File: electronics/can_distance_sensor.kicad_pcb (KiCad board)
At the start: 4 copper layers, 40.6 x 40.6 mm, 75 parts, among them J1 USB_B_Micro, J2 Conn_ARM_JTAG_SWD_10, J3 Conn_01x04, Q1 IRLML6401, SW1 PTS645SK50SMTR92LFS, U1 USBLC6-2SC6, U2 STM32G431CBUx, U3 TLV75801PDRV, U4 AOZ1280CI, U5 TLV75801PDRV, U6 TCAN1044A-Q1, U7 VL53L3CXV0DH/1, U8 TCA9509DGKR, Y1 Crystal_GND24

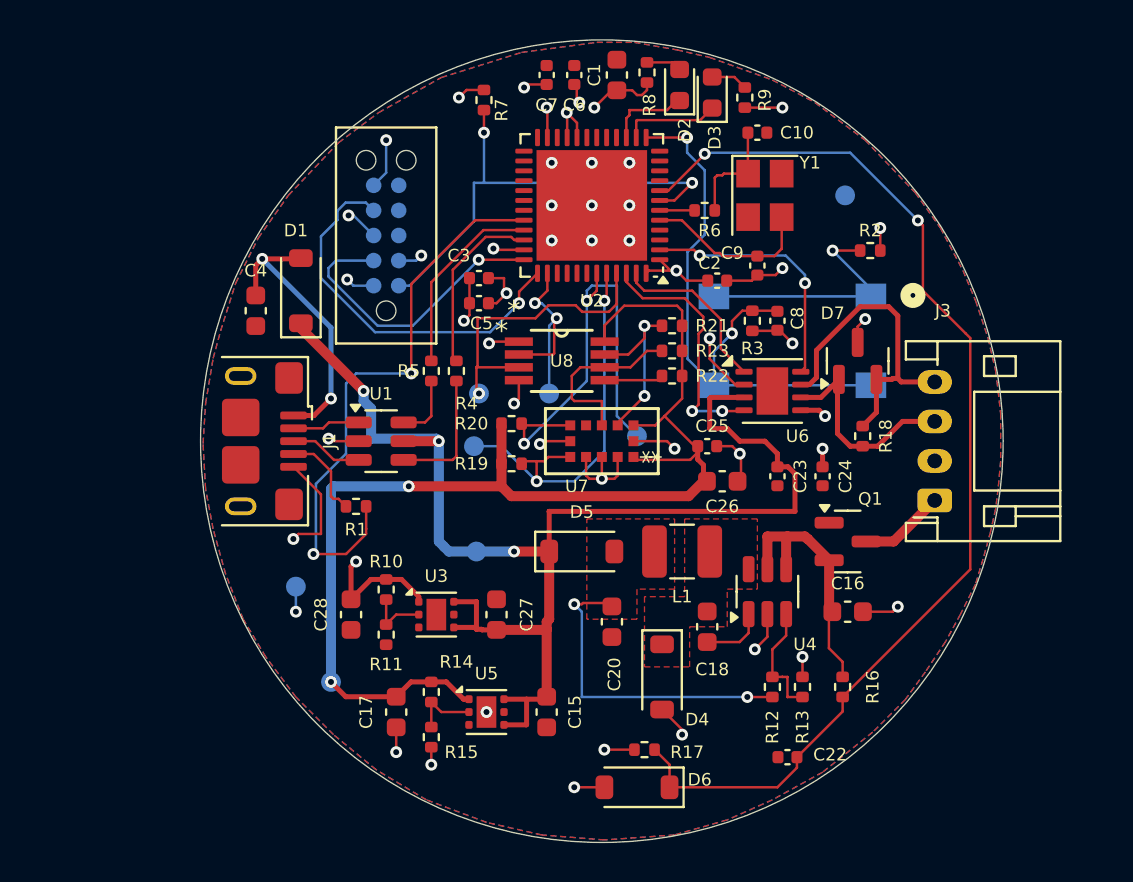
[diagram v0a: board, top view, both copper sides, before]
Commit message: Major refactor to rev B
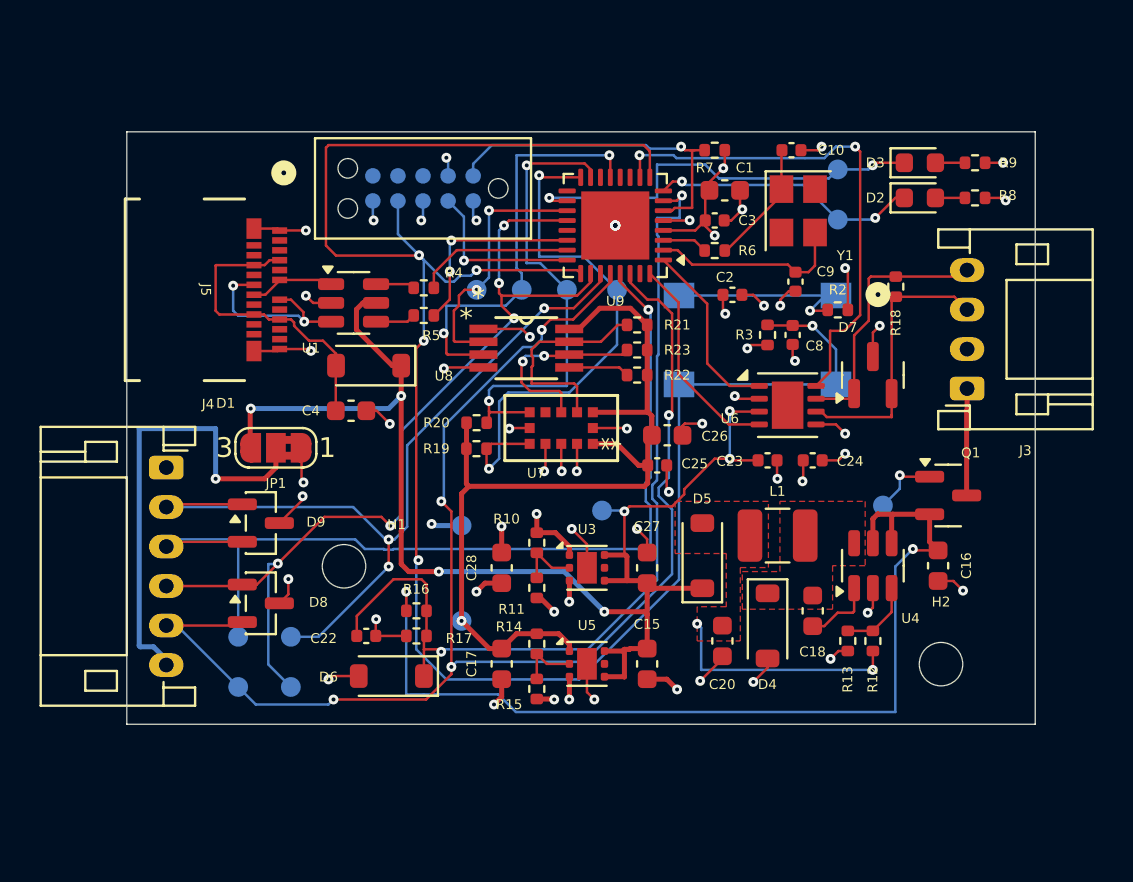
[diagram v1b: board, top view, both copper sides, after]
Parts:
- removed C5, C6, C7: 0.1u, Capacitor_SMD:C_0402_1005Metric
- removed J1: USB_B_Micro, Connector_USB:USB_Micro-B_Amphenol_10118193-0001LF_Horizontal
- removed R1: 560, Resistor_SMD:R_0402_1005Metric
- removed U2: STM32G431CBUx, Package_DFN_QFN:QFN-48-1EP_7x7mm_P0.5mm_EP5.6x5.6mm
- added D8: SP0502BAHT, Package_TO_SOT_SMD:SOT-23, F.Cu at (176.8, 113.9)
- added D9: SP0502BAHT, Package_TO_SOT_SMD:SOT-23, F.Cu at (176.8, 109.8)
- added H1: MountingHole, MountingHole:MountingHole_2.2mm_M2, F.Cu at (181.0, 112.0)
- added H2: MountingHole, MountingHole:MountingHole_2.2mm_M2, F.Cu at (211.2, 117.0)
- added J4: Conn_01x06, Connector_JST:JST_PH_S6B-PH-K_1x06_P2.00mm_Horizontal, F.Cu at (172.0, 107.0)
- added J5: USB_C_Receptacle, footprints:CONN_105450-0101_MOL, F.Cu at (174.0, 98.0)
- added JP1: SolderJumper_3_Bridged12, Jumper:SolderJumper-3_P1.3mm_Bridged2Bar12_RoundedPad1.0x1.5mm_NumberLabels, F.Cu at (177.6, 106.0)
- added TP10: TestPoint, TestPoint:TestPoint_Pad_D1.0mm, B.Cu at (175.6, 115.6)
- added TP11: TestPoint, TestPoint:TestPoint_Pad_D1.0mm, B.Cu at (175.6, 118.1)
- added TP12: TestPoint, TestPoint:TestPoint_Pad_D1.0mm, B.Cu at (178.3, 115.6)
- added TP13: TestPoint, TestPoint:TestPoint_Pad_D1.0mm, B.Cu at (206.0, 94.4)
- added TP14: TestPoint, TestPoint:TestPoint_Pad_D1.0mm, B.Cu at (206.0, 91.9)
- added TP9: TestPoint, TestPoint:TestPoint_Pad_D1.0mm, B.Cu at (178.3, 118.1)
- added U9: STM32G0B1KBUx, Package_DFN_QFN:QFN-32-1EP_5x5mm_P0.5mm_EP3.45x3.45mm, F.Cu at (194.7, 94.7)
- moved C22 22.2 mm to (182.1, 115.5), turned to 0 degrees
- moved TP8 22.1 mm to (190.0, 98.0)
- moved R16 21.9 mm to (184.7, 114.3), turned to 0 degrees
- moved TP1 21.2 mm to (208.3, 108.9), turned to 180 degrees
- moved TP6 20.4 mm to (192.3, 98.0)
- moved R8 17.8 mm to (213.0, 93.3), turned to 0 degrees
- moved D6 13.7 mm to (183.4, 117.6)
- moved D2 13.4 mm to (210.2, 93.3), turned to 0 degrees
- moved TP7 13.3 mm to (187.7, 98.0)
- moved R17 12.9 mm to (184.7, 115.5)
- moved TP5 12.5 mm to (194.8, 98.0), turned to 180 degrees
- moved C3 12.3 mm to (199.8, 94.5), turned to 0 degrees
- moved R9 12.1 mm to (213.0, 91.6), turned to 0 degrees
- moved R7 12.0 mm to (199.8, 90.9), turned to 0 degrees
- moved D3 11.1 mm to (210.2, 91.6), turned to 0 degrees
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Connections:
- D7 pad 1: Net-(J3-Pin_3) -> Net-(J3-Pin_4)
- D7 pad 2: Net-(J3-Pin_4) -> Net-(J3-Pin_3)
- J2 pad 4: SWCLK -> BOOT
- TP1 pad 1: TOF_SDA -> GND
- TP2 pad 1: TOF_SCL -> VCC
- TP3 pad 1: TOF_INT -> 3V3
- TP4 pad 1: TOF_XSHUT -> 2V8
- TP5 pad 1: GND -> TOF_XSHUT
- TP6 pad 1: 3V3 -> TOF_INT
- TP7 pad 1: VCC -> TOF_SCL
- TP8 pad 1: 2V8 -> TOF_SDA
- U1 pad 4: Net-(R4-Pad1) -> Net-(R5-Pad1)
- U1 pad 6: Net-(R5-Pad1) -> Net-(R4-Pad1)
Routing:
- net TB_ABS: track 0.00 -> 75.8 mm, vias 0 -> 5
- net BOOT: track 30.0 -> 100.0 mm, vias 2 -> 5
- net TB_MOSI: track 0.00 -> 48.6 mm, vias 0 -> 1
- net TB_CS: track 0.00 -> 46.9 mm, vias 0 -> 5
- net TB_CLK: track 0.00 -> 42.6 mm, vias 0 -> 3
- net +12V: track 13.2 -> 49.0 mm, vias 0 -> 2
- net ID: track 28.9 -> 0.00 mm, vias 2 -> 0
- net Net-(J4-Pin_6): track 0.00 -> 23.6 mm, vias 0 -> 1
- net GND: track 49.1 -> 69.9 mm, vias 33 -> 53
- net SWCLK: track 19.6 -> 0.00 mm, vias 1 -> 0
- net LED2: track 4.96 -> 21.2 mm, vias 0 -> 2
- net 2V8: track 61.0 -> 45.2 mm, vias 2 -> 1
- net CAN_STB: track 12.9 -> 25.9 mm
- net VIN_MEAS: track 56.8 -> 45.5 mm
- net LED1: track 4.26 -> 13.6 mm, vias 0 -> 2
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- removed copper zone on B.Cu, net GND
- removed copper zone on F.Cu, net GND
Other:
- board size 40.6 x 40.6 mm -> 46 x 30 mm
- board text added: "TOF Utility Rev B Copyright 2025 Team 7048 & 4360"
- board text added: "TP1 = GND TP2 = +5V TP3 = +3.3V TP4 = 2.8V TP5 = TOF_XSHUT TP6 = TOF_INT TP7 = TOF_SCL TP8 = TOF_SDA TP9 = TB_CS TP10 = TB_MOSI TP11 = TB_MISO TP12 = TB_CLK"
- board text removed: "I'm Not Touching You Rev A Copyright 2024 Team 7048 & 4360"
- board text removed: "TP1 = 3.3V TP2 = TOF_SDA TP3 = VCC TP4 = TOF_SCL TP5 = TOF_INT TP6 = TOF_XSHUT TP7 = GND"
